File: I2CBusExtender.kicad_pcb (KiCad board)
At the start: 2 copper layers, 57.5 x 17.9 mm, 19 parts, among them J1 SBusConn, J2 LBusCon, U1 P82B715

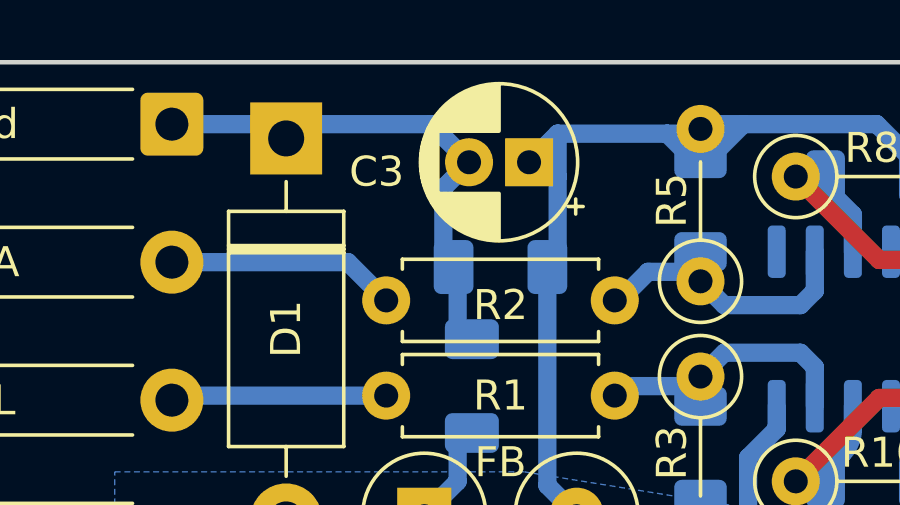
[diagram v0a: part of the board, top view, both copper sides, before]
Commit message: Tweaked track layout.
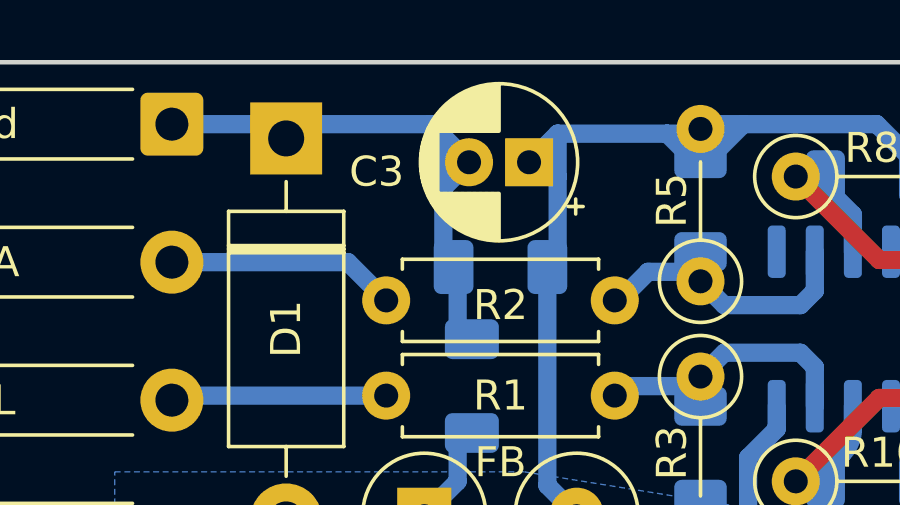
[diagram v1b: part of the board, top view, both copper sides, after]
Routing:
- net /Gnd: track 20.2 -> 22.0 mm
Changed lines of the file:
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@@
   (segment (start 91.7575 92.55125) (end 91.7575 94.4325) (width 0.6096) (layer "B.Cu") (net 3))
   (via (at 108.10875 93.18625) (size 1.28) (drill 0.7) (layers "F.Cu" "B.Cu") (net 4))
+  (segment (start 96.99625 79.7875) (end 96.99625 81.5025) (width 0.6096) (layer "B.Cu") (net 4))
+  (segment (start 108.10875 88.77625) (end 108.10875 89.535) (width 0.6096) (layer "B.Cu") (net 4))
   (segment (start 92.86875 79.375) (end 96.58375 79.375) (width 0.6096) (layer "B.Cu") (net 4))
-  (segment (start 108.10875 88.77625) (end 108.10875 89.535) (width 0.6096) (layer "B.Cu") (net 4))
-  (segment (start 96.58375 79.375) (end 97.85375 80.645) (width 0.6096) (layer "B.Cu") (net 4))
-  (segment (start 97.85375 80.645) (end 96.99625 81.5025) (width 0.6096) (layer "B.Cu") (net 4))
   (segment (start 108.10875 89.535) (end 107.15625 90.4875) (width 0.6096) (layer "B.Cu") (net 4))
   (segment (start 91.28125 79.375) (end 91.7575 79.85125) (width 0.6096) (layer "B.Cu") (net 4))
-  (segment (start 96.99625 81.5025) (end 96.99625 83.66125) (width 0.6096) (layer "B.Cu") (net 4))
+  (segment (start 96.99625 81.5025) (end 96.99625 83.795) (width 0.6096) (layer "B.Cu") (net 4))
   (segment (start 107.15625 92.23375) (end 108.10875 93.18625) (width 0.6096) (layer "B.Cu") (net 4))
   (segment (start 107.15625 90.4875) (end 107.15625 92.23375) (width 0.6096) (layer "B.Cu") (net 4))
   (segment (start 87.9475 79.375) (end 91.28125 79.375) (width 0.6096) (layer "B.Cu") (net 4))
+  (segment (start 97.85375 80.645) (end 96.99625 81.5025) (width 0.6096) (layer "B.Cu") (net 4))
+  (segment (start 96.58375 79.375) (end 96.99625 79.7875) (width 0.6096) (layer "B.Cu") (net 4))
+  (segment (start 96.99625 79.7875) (end 97.85375 80.645) (width 0.6096) (layer "B.Cu") (net 4))
   (segment (start 97.4725 86.54375) (end 97.4725 84.455) (width 0.6096) (layer "B.Cu") (net 4))
   (segment (start 93.8175 83.975) (end 95.09125 85.24875) (width 0.6096) (layer "B.Cu") (net 5))
